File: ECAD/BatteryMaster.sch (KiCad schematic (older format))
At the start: 45 parts

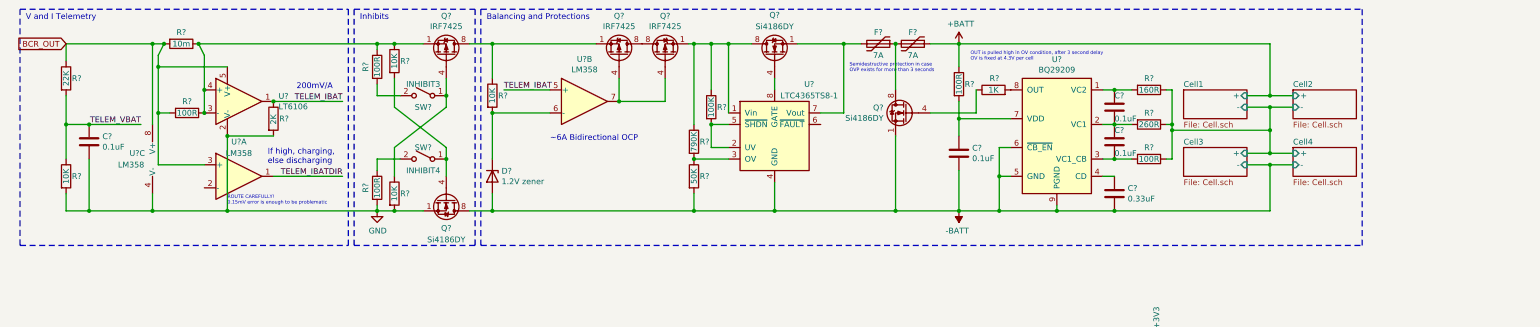
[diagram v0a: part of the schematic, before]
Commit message: bidirectional inhibits, remove unrealistic zener, replace all irf7425 with irf7458
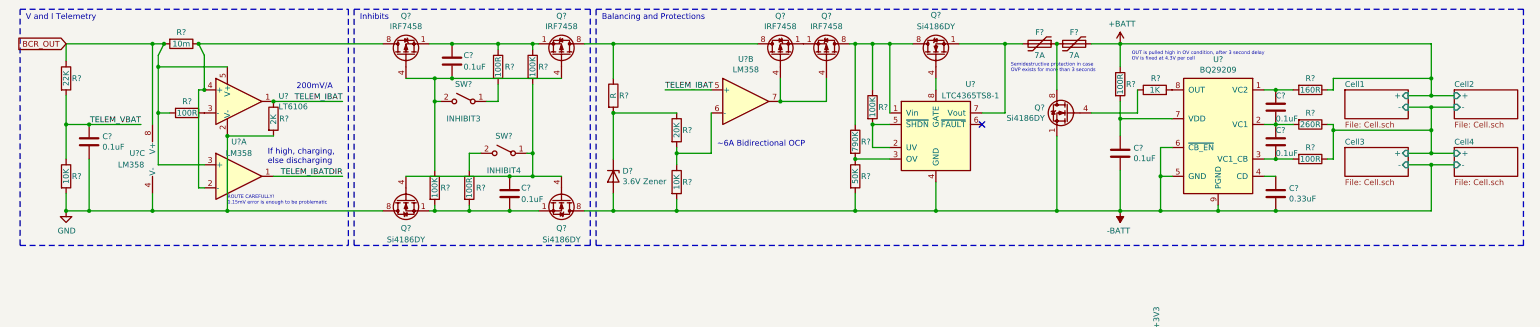
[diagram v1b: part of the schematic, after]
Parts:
- removed R? (x2): 10K, symbol Device:R
- added C? (x2): 0.1uF, symbol Device:C
- added Q?: IRF7458, Package_SO:SOIC-8_3.9x4.9mm_P1.27mm, symbol Transistor_FET:IRF7404
- added Q?: Si4186DY, Package_SO:SOIC-8_3.9x4.9mm_P1.27mm, symbol Transistor_FET:Si4162DY
- added R? (x2): 100K, symbol Device:R
- added R?: 20K, symbol Device:R
- added R?: 10K, symbol Device:R
- D?: value 1.2V zener -> 3.6V Zener
- Q? (x3): value IRF7425 -> IRF7458
- R?: value 10K -> R
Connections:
- net +BATT: now also R?.1
- net -BATT: now also Q?.5 (D), Q?.6 (D), Q?.7 (D), Q?.8 (D), R?.2; no longer Q?.5 (D), Q?.6 (D), Q?.7 (D), Q?.8 (D)
- net Cell1/-: no longer R?.1
- net GND: now also Q?.5 (D), Q?.6 (D), Q?.7 (D), Q?.8 (D); no longer Q?.1 (S), Q?.2 (S), Q?.3 (S), R?.2
- net at Q?.4 (G), SW?.1 (A): now also C?.1, Q?.4 (G), R?.2
- net at Q?.1 (S), Q?.2 (S), Q?.3 (S)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: now also C?.1, Q?.1 (S), Q?.2 (S), Q?.3 (S), R?.1; no longer R?.1, R?.1, U?.3 (-), U?.4 (+)
- net at Q?.4 (G): now also SW?.2 (B), C?.2, Q?.4 (G), R?.1; no longer SW?.1 (A)
- net at Q?.5 (D), Q?.6 (D), Q?.7 (D)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: now also R?.1, U?.2 (-), U?.4 (+); no longer Q?.1 (S), Q?.2 (S), Q?.3 (S), R?.1
- net at Q?.5 (D), Q?.6 (D), Q?.7 (D)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: now also Q?.5 (D), Q?.6 (D), Q?.7 (D), Q?.8 (D); no longer Q?.1 (S), Q?.2 (S), Q?.3 (S)
- net at Q?.5 (D), Q?.6 (D), Q?.7 (D)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: now also R?.1, Q?.5 (D), Q?.6 (D), Q?.7 (D), Q?.8 (D); no longer Q?.5 (D), Q?.6 (D), Q?.7 (D), Q?.8 (D)
- net at R?.2: now also SW?.1 (A); no longer SW?.2 (B)
- net at D?.1 (K), R?.2: now also R?.1; no longer U?.6 (-)
- new net: C?.2, Q?.1 (S), Q?.1 (S), Q?.2 (S), Q?.2 (S), Q?.3 (S), Q?.3 (S), R?.2, R?.2
- new net: Q?.1 (S), Q?.1 (S), Q?.2 (S), Q?.2 (S), Q?.3 (S), Q?.3 (S)
- new net: R?.1, U?.3 (-)
- new net: R?.1, R?.2, U?.6 (-)
- no-connect marks 16 -> 17
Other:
- moved on the sheet: C?, D?, F?, Q?, R?, SW?, U?, U?B
